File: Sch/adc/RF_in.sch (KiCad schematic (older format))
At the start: 63 parts, among them J3 JP2, J4 JP2, U1 LTC2292, U2 BGA2818, U3 TLV711, X1 ECS-TXO-2520

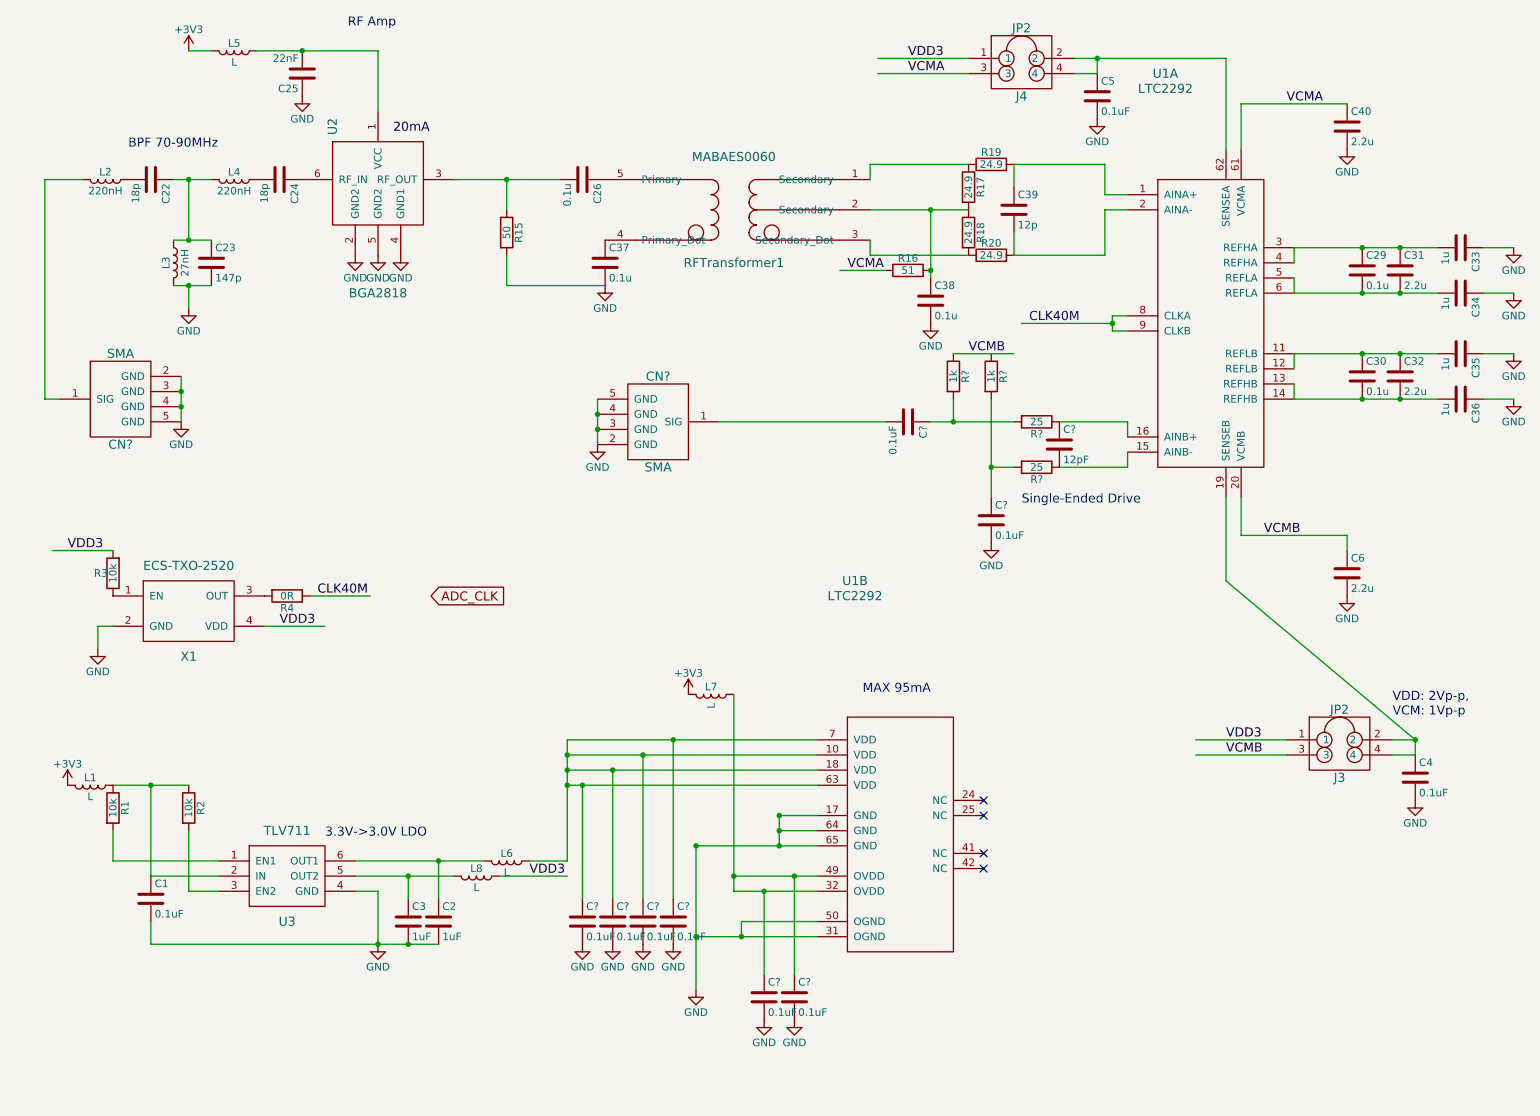
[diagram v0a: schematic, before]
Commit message: Almost finished except Audio
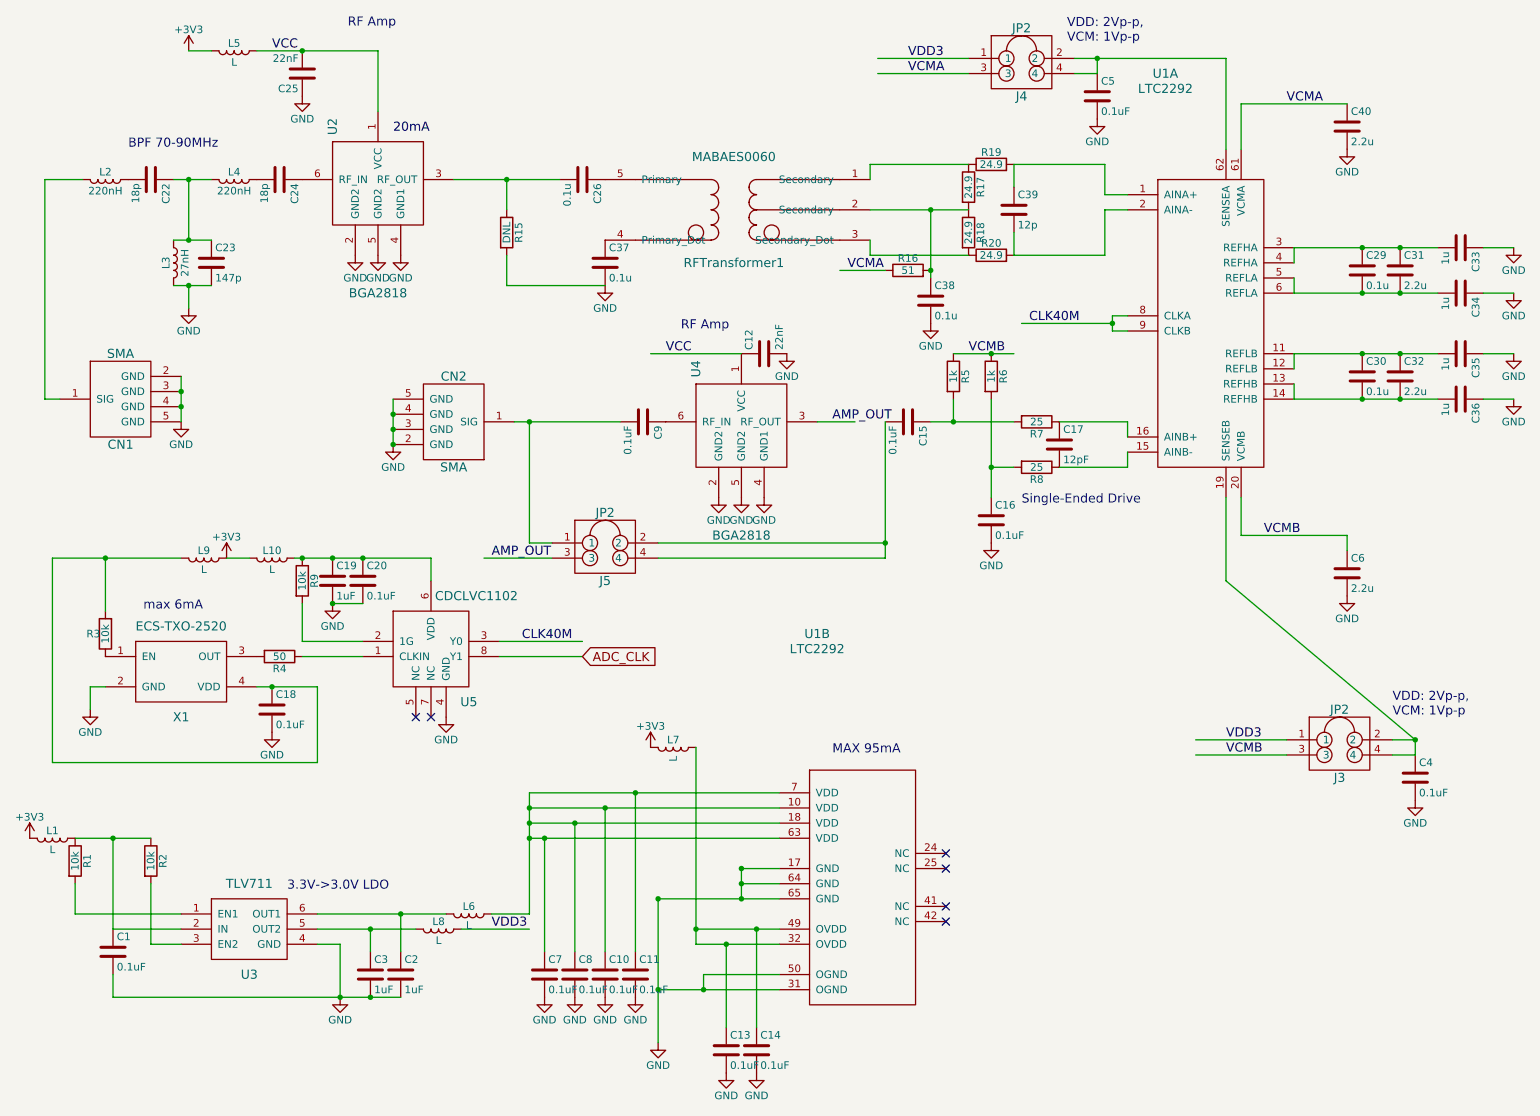
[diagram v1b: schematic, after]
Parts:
- added C12: 22nF, symbol C
- added C18, C20, C9: 0.1uF, symbol C
- added C19: 1uF, symbol C
- added J5: JP2, symbol JP2
- added L10, L9: L, symbol L
- added R9: 10k, symbol R
- added U4: BGA2818, symbol BGA2818
- added U5: CDCLVC1102, symbol CDCLVC1102
- R15: value 50 -> DNL
- R4: value 0R -> 50
- gave numbers to parts that had none: 15
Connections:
- net labels added: AMP_OUT, VCC
- wire segments 120 -> 140
- no-connect marks 4 -> 6
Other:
- note added: "max 6mA"
- moved on the sheet: C1, C10, C11, C13, C14, C2, C3, C7, C8, CN2, L1, L6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
